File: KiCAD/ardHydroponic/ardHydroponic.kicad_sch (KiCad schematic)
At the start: 29 parts, among them J1 LCD display, J2 Buttons, J3 MOSFETs, K1 KY-019_relay_module, SW1 button1, SW2 button2, SW3 button3, SW4 button4, SW5 button5, U1 DS18B20, U10 ESP-01, U2 pH sensor, U3 TDS meter, U4 Power in, U5 pH+ pump, U6 pH- pump, U7 nutr A pump, U8 nutr B pump, U9 stirrer

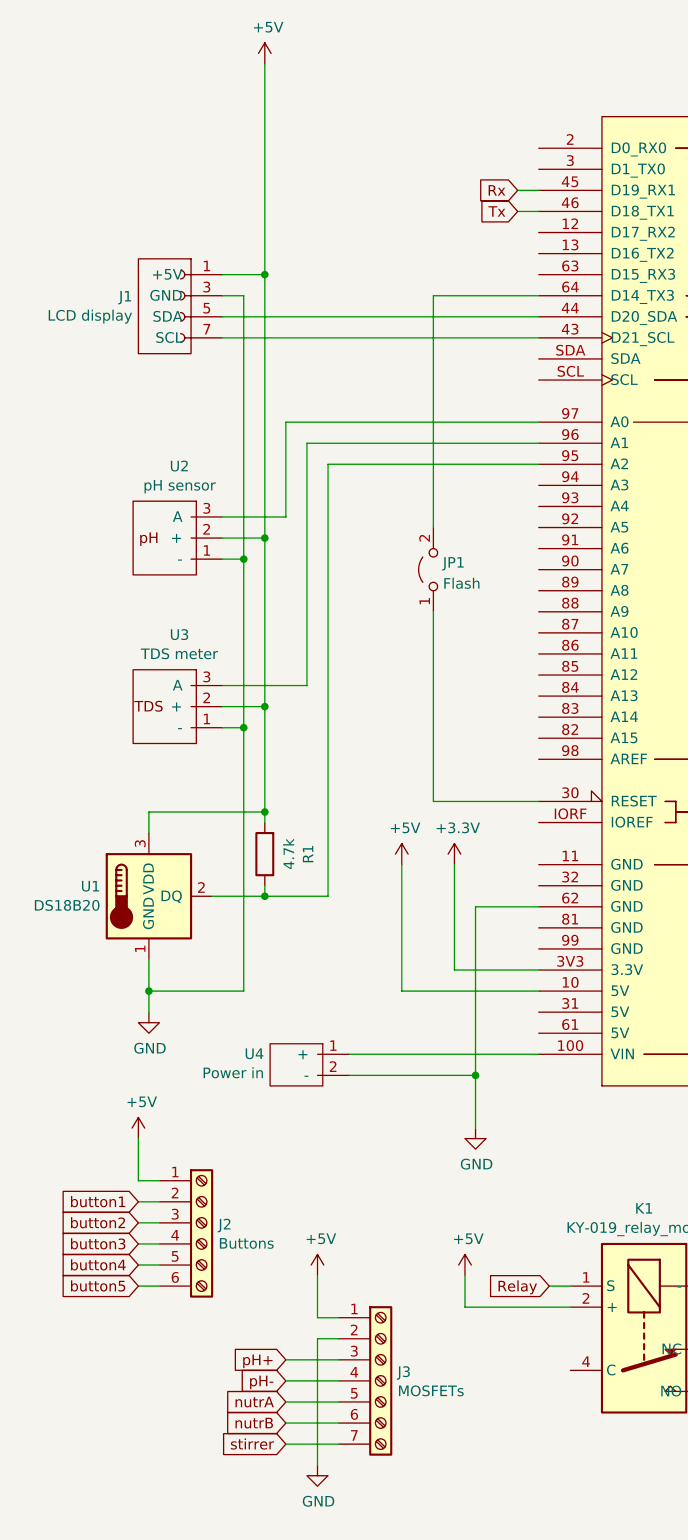
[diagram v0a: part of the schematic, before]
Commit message: new pcb
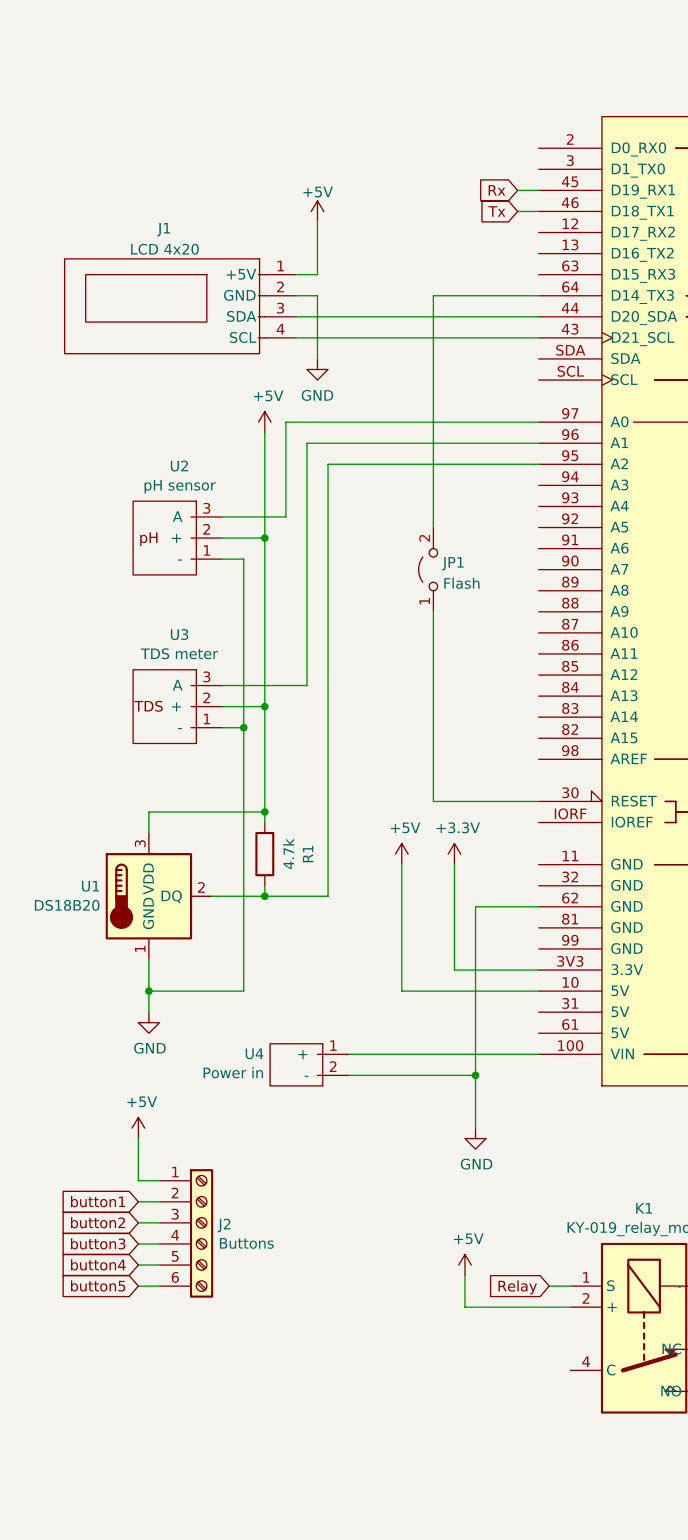
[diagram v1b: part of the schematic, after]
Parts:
- removed J3: MOSFETs, My_Parts:7-pole_6-MOSFET_screw_terminal, symbol Connector:Screw_Terminal_01x07
- J1: value LCD display -> LCD 4x20; footprint My_Headers:4-pin_I2C_LCD_header_larger -> My_Headers:4-pin JST LCD
- J2: footprint My_Parts:6-pole_5-NO_switch_screw_terminal -> My_Headers:6-pin JST 5-buttons
- K1: footprint My_Headers:3-pin_KY-019_Relay_header_larger_pads -> My_Headers:3-pin JST KY-019 relay
- U1: footprint My_Parts:3-pole_DS18B20_screw_terminal -> My_Headers:3-pin JST DS18B20
- U2: footprint My_Headers:3-pin_DFRobot_Gravity_pH-sensor_header_large -> My_Headers:3-pin JST pH Sensor
- U3: footprint My_Headers:3-pin_DFRobot_Gravity_TDS-meter_header_large -> My_Headers:3-pin JST TDS Meter
- U5, U6, U7, U8, U9: footprint (none) -> My_Headers:3-pin JST IRF520 MOSFET module
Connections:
- net GND: now also J1.2 (GND); no longer J1.3 (GND)
- net at XA1.43 (D21_SCL): now also J1.4 (SCL); no longer J1.7 (SCL)
- net at XA1.44 (D20_SDA): now also J1.3 (SDA); no longer J1.5 (SDA)
